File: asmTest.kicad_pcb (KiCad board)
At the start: 2 copper layers, 3 parts, among them U1 LM5109ASD, U2 LM5109ASD, U3 LM5109ASD

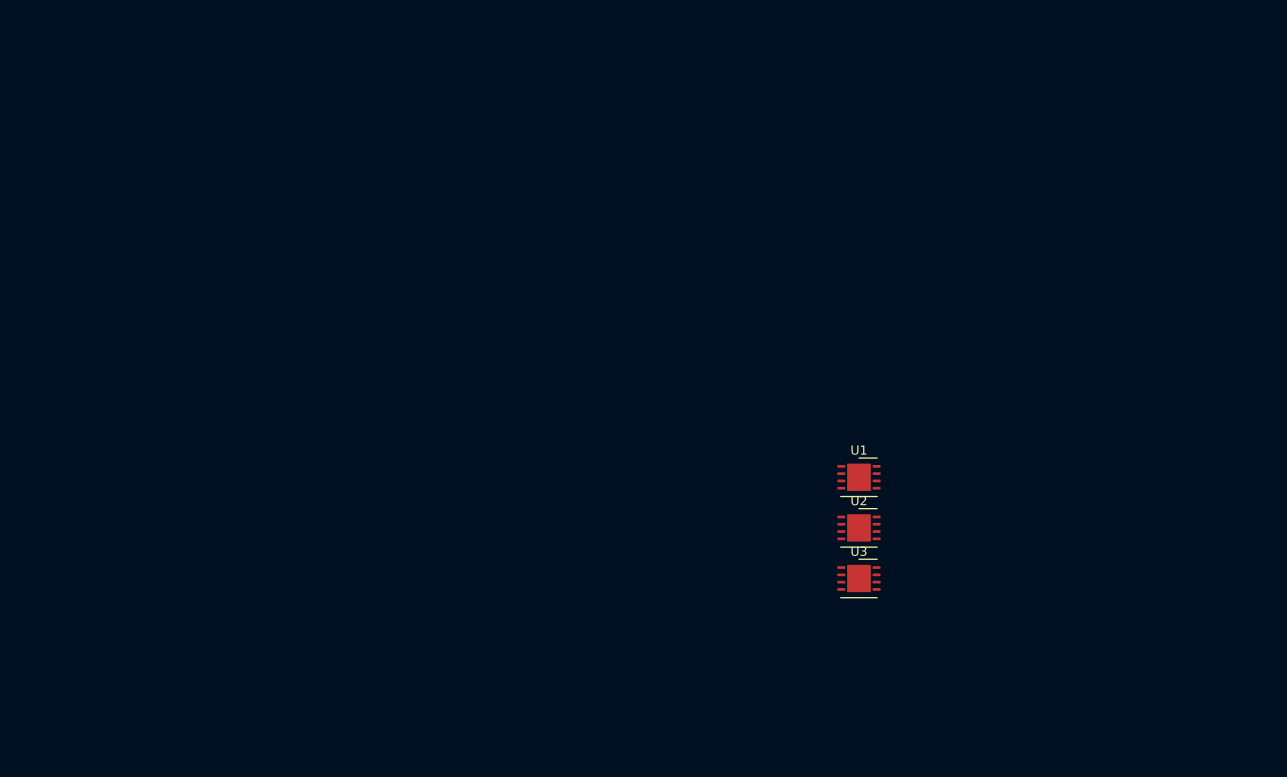
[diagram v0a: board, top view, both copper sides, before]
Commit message: first iteration of test
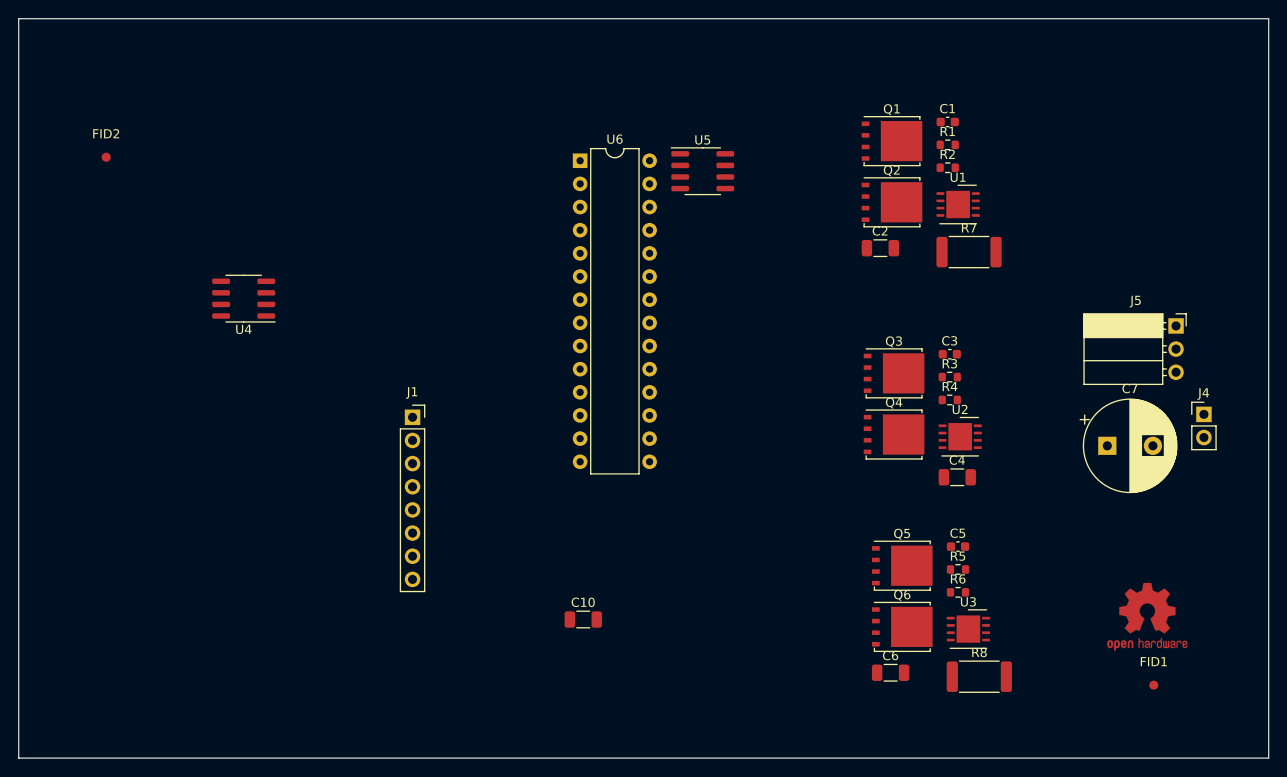
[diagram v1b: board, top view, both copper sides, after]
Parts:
- added C1: 100n, Capacitor_SMD:C_0603_1608Metric, F.Cu at (186.7, 48.6)
- added C10: 2u2, Capacitor_SMD:C_1206_3216Metric, F.Cu at (146.7, 103.2)
- added C2: 1u, Capacitor_SMD:C_1206_3216Metric, F.Cu at (179.3, 62.5)
- added C3: 100n, Capacitor_SMD:C_0603_1608Metric, F.Cu at (186.9, 74.1)
- added C4: 1u, Capacitor_SMD:C_1206_3216Metric, F.Cu at (187.7, 87.6)
- added C5: 100n, Capacitor_SMD:C_0603_1608Metric, F.Cu at (187.8, 95.2)
- added C6: 1u, Capacitor_SMD:C_1206_3216Metric, F.Cu at (180.4, 109.0)
- added C7: 100u/100V, Capacitor_THT:CP_Radial_D10.0mm_P5.00mm, F.Cu at (204.2, 84.2)
- added FID1: Fiducial, Fiducial:Fiducial_1mm_Mask3mm, F.Cu at (209.3, 110.4)
- added FID2: Fiducial, Fiducial:Fiducial_1mm_Mask3mm, F.Cu at (94.4, 52.5)
- added J1: Conn_01x08_Pin, Connector_PinSocket_2.54mm:PinSocket_1x08_P2.54mm_Vertical, F.Cu at (128.0, 81.0)
- added J4: Conn_01x02_Pin, Connector_PinHeader_2.54mm:PinHeader_1x02_P2.54mm_Vertical, F.Cu at (214.8, 80.7)
- added J5: Conn_01x03_Socket, Connector_PinSocket_2.54mm:PinSocket_1x03_P2.54mm_Horizontal, F.Cu at (211.7, 71.0)
- added LOGO1: var1, Symbol:OSHW-Logo2_9.8x8mm_Copper, F.Cu at (208.6, 102.9)
- added Q1: BSC026N08, Package_TO_SOT_SMD:TDSON-8-1, F.Cu at (180.6, 50.7)
- added Q2: BSC026N08, Package_TO_SOT_SMD:TDSON-8-1, F.Cu at (180.6, 57.4)
- added Q3: BSC026N08, Package_TO_SOT_SMD:TDSON-8-1, F.Cu at (180.8, 76.2)
- added Q4: BSC026N08, Package_TO_SOT_SMD:TDSON-8-1, F.Cu at (180.8, 82.9)
- added Q5: BSC026N08, Package_TO_SOT_SMD:TDSON-8-1, F.Cu at (181.7, 97.3)
- added Q6: BSC026N08, Package_TO_SOT_SMD:TDSON-8-1, F.Cu at (181.7, 104.0)
- added R1: 33R, Resistor_SMD:R_0603_1608Metric, F.Cu at (186.7, 51.1)
- added R2: 33R, Resistor_SMD:R_0603_1608Metric, F.Cu at (186.7, 53.6)
- added R3: 33R, Resistor_SMD:R_0603_1608Metric, F.Cu at (186.9, 76.6)
- added R4: 33R, Resistor_SMD:R_0603_1608Metric, F.Cu at (186.9, 79.1)
- added R5: 33R, Resistor_SMD:R_0603_1608Metric, F.Cu at (187.8, 97.7)
- added R6: 33R, Resistor_SMD:R_0603_1608Metric, F.Cu at (187.8, 100.2)
- added R7: 0.001R, Resistor_SMD:R_2512_6332Metric, F.Cu at (189.0, 62.9)
- added R8: 0.001R, Resistor_SMD:R_2512_6332Metric, F.Cu at (190.2, 109.5)
- added U4: SN65HVD1050D, Package_SO:SOIC-8_3.9x4.9mm_P1.27mm, F.Cu at (109.5, 68.0)
- added U5: ADuM121N, Package_SO:SOIC-8_3.9x4.9mm_P1.27mm, F.Cu at (159.8, 54.0)
- added U6: ATmega328P-P, Package_DIP:DIP-28_W7.62mm, F.Cu at (146.4, 52.9)
- U1, U2, U3: value LM5109ASD -> LM5109BSD
- moved U1 31.8 mm to (187.8, 57.7)
- moved U2 14.9 mm to (188.1, 83.2)
- moved U3 13.2 mm to (189.0, 104.2)
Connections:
- U1 pad 1: unconnected-(U1-VDD-Pad1) -> +10V
- U1 pad 2: unconnected-(U1-HI-Pad2) -> /hi_A
- U1 pad 3: unconnected-(U1-LI-Pad3) -> /li_A
- U1 pad 4: Net-(U1-VSS-Pad4) -> GND
- U1 pad 5: unconnected-(U1-LO-Pad5) -> Net-(U1-LO)
- U1 pad 6: unconnected-(U1-HS-Pad6) -> Net-(Q2-D)
- U1 pad 7: unconnected-(U1-HO-Pad7) -> Net-(U1-HO)
- U1 pad 8: unconnected-(U1-HB-Pad8) -> Net-(U1-HB)
- U1 pad 9: Net-(U1-VSS-Pad4) -> GND
- U2 pad 1: unconnected-(U2-VDD-Pad1) -> +10V
- U2 pad 2: unconnected-(U2-HI-Pad2) -> /hi_B
- U2 pad 3: unconnected-(U2-LI-Pad3) -> /li_B
- U2 pad 4: Net-(U2-VSS-Pad4) -> GND
- U2 pad 5: unconnected-(U2-LO-Pad5) -> Net-(U2-LO)
- U2 pad 6: unconnected-(U2-HS-Pad6) -> /phase_B
- U2 pad 7: unconnected-(U2-HO-Pad7) -> Net-(U2-HO)
- U2 pad 8: unconnected-(U2-HB-Pad8) -> Net-(U2-HB)
- U2 pad 9: Net-(U2-VSS-Pad4) -> GND
- U3 pad 1: unconnected-(U3-VDD-Pad1) -> +10V
- U3 pad 2: unconnected-(U3-HI-Pad2) -> /hi_C
- U3 pad 3: unconnected-(U3-LI-Pad3) -> /li_C
- U3 pad 4: Net-(U3-VSS-Pad4) -> GND
- U3 pad 5: unconnected-(U3-LO-Pad5) -> Net-(U3-LO)
- U3 pad 6: unconnected-(U3-HS-Pad6) -> Net-(Q6-D)
- U3 pad 7: unconnected-(U3-HO-Pad7) -> Net-(U3-HO)
- U3 pad 8: unconnected-(U3-HB-Pad8) -> Net-(U3-HB)
- U3 pad 9: Net-(U3-VSS-Pad4) -> GND
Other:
- board outline added: 137.1 x 81.1 mm
